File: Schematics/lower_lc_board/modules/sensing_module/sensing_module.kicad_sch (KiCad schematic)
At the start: 21 parts, among them J4 HALL-1, J5 HALL-2, Q3 2N7002, U11 SI2301CDS-T1-GE3, U9 ADC_ADS131M04IPWR

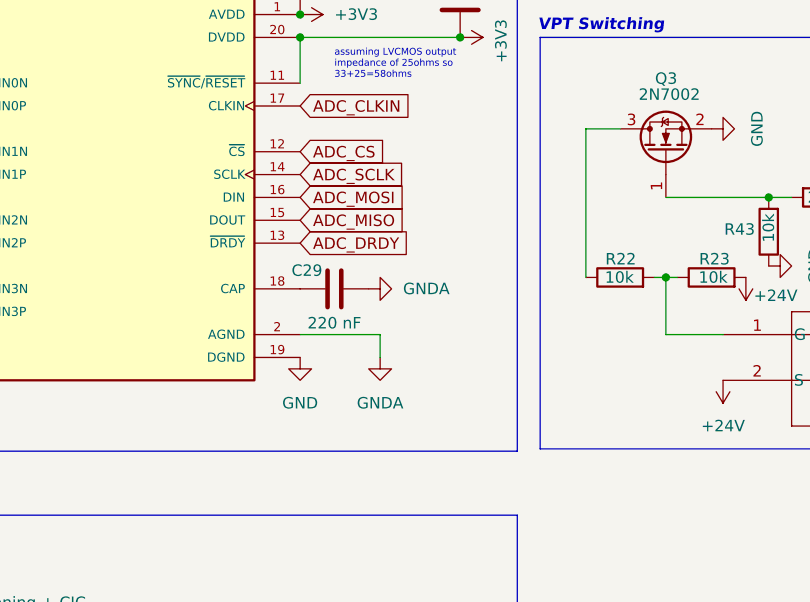
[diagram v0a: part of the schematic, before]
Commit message: routing work
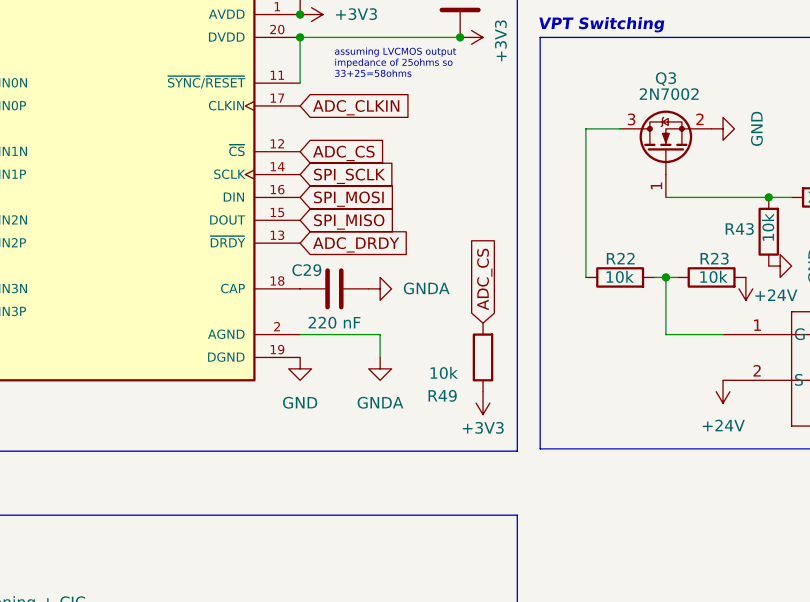
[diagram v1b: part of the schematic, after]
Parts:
- added R49: 10k, Resistor_SMD:R_0402_1005Metric, symbol Device:R
- C23, C33: JLCPCB (none) -> C49678
- J4, J5: footprint B04B_PASK_JST:CONN_B04B-PASK_JST -> S04B_PASK_2-P:CONN4_S04B-PASK_JST
- R22, R23: JLCPCB (none) -> C25744
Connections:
- net +3V3: now also R49.1
- net ADC_CS: now also R49.2
- net ADC_MISO renamed SPI_MISO
- net ADC_MOSI renamed SPI_MOSI
- net ADC_SCLK renamed SPI_SCLK
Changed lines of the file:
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@@
 		)
 	)
-	(global_label "ADC_DRDY"
+	(global_label "SPI_MISO"
 		(shape input)
-		(at 182.88 69.85 0)
+		(at 182.88 67.31 0)
 		(fields_autoplaced yes)
 		(effects
@@
 		)
 		(property "Intersheetrefs" "${INTERSHEET_REFS}"
-			(at 195.36 69.85 0)
+			(at 194.5133 67.31 0)
 			(effects
 				(font
@@
 		)
 	)
-	(global_label "HALL_SCL"
+	(global_label "ADC_DRDY"
 		(shape input)
-		(at 91.44 139.7 180)
+		(at 182.88 69.85 0)
 		(fields_autoplaced yes)
 		(effects
@@
 				(size 1.27 1.27)
 			)
-			(justify right)
+			(justify left)
 		)
 		(property "Intersheetrefs" "${INTERSHEET_REFS}"
-			(at 79.5043 139.7 0)
+			(at 195.36 69.85 0)
 			(effects
 				(font
 					(size 1.27 1.27)
 				)
-				(justify right)
+				(justify left)
 				(hide yes)
 			)
 		)
 	)
-	(global_label "ADC_CS"
+	(global_label "HALL_SCL"
 		(shape input)
-		(at 182.88 59.69 0)
+		(at 91.44 139.7 180)
 		(fields_autoplaced yes)
 		(effects
@@
 				(size 1.27 1.27)
 			)
-			(justify left)
+			(justify right)
 		)
 		(property "Intersheetrefs" "${INTERSHEET_REFS}"
-			(at 192.9409 59.69 0)
+			(at 79.5043 139.7 0)
 			(effects
 				(font
 					(size 1.27 1.27)
 				)
-				(justify left)
+				(justify right)
 				(hide yes)
 			)
 		)
 	)
-	(global_label "ADC_SCLK"
+	(global_label "ADC_CS"
 		(shape input)
-		(at 182.88 62.23 0)
+		(at 182.88 59.69 0)
 		(fields_autoplaced yes)
 		(effects
@@
 		)
 		(property "Intersheetrefs" "${INTERSHEET_REFS}"
-			(at 195.239 62.23 0)
+			(at 192.9409 59.69 0)
 			(effects
 				(font
@@
 		)
 	)
-	(global_label "ADC_MOSI"
+	(global_label "ADC_CLKIN"
 		(shape input)
-		(at 182.88 64.77 0)
+		(at 182.88 54.61 0)
 		(fields_autoplaced yes)
 		(effects
@@
 		)
 		(property "Intersheetrefs" "${INTERSHEET_REFS}"
-			(at 195.0576 64.77 0)
+			(at 195.9648 54.61 0)
 			(effects
 				(font
@@
 		)
 	)
-	(global_label "ADC_CLKIN"
+	(global_label "ADC_CS"
 		(shape input)
-		(at 182.88 54.61 0)
+		(at 203.2 78.74 90)
 		(fields_autoplaced yes)
 		(effects
@@
 		)
 		(property "Intersheetrefs" "${INTERSHEET_REFS}"
-			(at 195.9648 54.61 0)
+			(at 203.2 68.6791 90)
 			(effects
 				(font
@@
 		)
 	)
-	(global_label "ADC_MISO"
+	(global_label "SPI_SCLK"
 		(shape input)
-		(at 182.88 67.31 0)
+		(at 182.88 62.23 0)
 		(fields_autoplaced yes)
 		(effects
@@
 		)
 		(property "Intersheetrefs" "${INTERSHEET_REFS}"
-			(at 195.0576 67.31 0)
+			(at 194.6947 62.23 0)
 			(effects
 				(font
@@
 		)
 	)
+	(global_label "SPI_MOSI"
+		(shape input)
+		(at 182.88 64.77 0)
+		(fields_autoplaced yes)
+		(effects
+			(font
+				(size 1.27 1.27)
+			)
+			(justify left)
+		)
+		(property "Intersheetrefs" "${INTERSHEET_REFS}"
+			(at 194.5133 64.77 0)
+			(effects
+				(font
+					(size 1.27 1.27)
+				)
+				(justify left)
+				(hide yes)
+			)
+		)
+	)
 	(symbol
 		(lib_id "Device:C")
@@
 			)
 		)
+		(property "JLCPCB" "C25744"
+			(at 228.6 73.66 0)
+			(effects
+				(font
+					(size 1.27 1.27)
+				)
+				(hide yes)
+			)
+		)
 		(pin "1"
 		)
@@
 			)
 		)
+		(property "JLCPCB" "C49678"
+			(at 45.72 170.18 0)
+			(effects
+				(font
+					(size 1.27 1.27)
+				)
+				(hide yes)
+			)
+		)
 		(pin "2"
 		)
@@
 			)
 		)
-		(property "Footprint" "B04B_PASK_JST:CONN_B04B-PASK_JST"
+		(property "Footprint" "S04B_PASK_2-P:CONN4_S04B-PASK_JST"
 			(at 49.53 154.94 0)
 			(effects
@@
 			)
 		)
+		(property "JLCPCB" "C49678"
+			(at 45.72 130.81 0)
+			(effects
+				(font
+					(size 1.27 1.27)
+				)
+				(hide yes)
+			)
+		)
 		(pin "2"
 		)
@@
 	)
 	(symbol
+		(lib_id "power:+3V3")
+		(at 203.2 86.36 180)
+		(unit 1)
+		(exclude_from_sim no)
+		(in_bom yes)
+		(on_board yes)
+		(dnp no)
+		(property "Reference" "#PWR0132"
+			(at 203.2 82.55 0)
+			(effects
+				(font
+					(size 1.27 1.27)
+				)
+				(hide yes)
+			)
+		)
+		(property "Value" "+3V3"
+			(at 203.2 90.424 0)
+			(effects
+				(font
+					(size 1.27 1.27)
+				)
+			)
+		)
+		(property "Footprint" ""
+			(at 203.2 86.36 0)
+			(effects
+				(font
+					(size 1.27 1.27)
+				)
+				(hide yes)
+			)
+		)
+		(property "Datasheet" ""
+			(at 203.2 86.36 0)
+			(effects
+				(font
+					(size 1.27 1.27)
+				)
+				(hide yes)
+			)
+		)
+		(property "Description" "Power symbol creates a global label with name \"+3V3\""
+			(at 203.2 86.36 0)
+			(effects
+				(font
+					(size 1.27 1.27)
+				)
+				(hide yes)
+			)
+		)
+		(pin "1"
+		)
+		(instances
+			(project "lower_lc_board"
+				(path "/d63798c4-e363-437e-9012-e4aff32e6642/c6419db7-28a9-4bfa-8244-fc88166c795c"
+					(reference "#PWR0132")
+					(unit 1)
+				)
+			)
+		)
+	)
+	(symbol
 		(lib_id "Device:C")
 		(at 186.69 74.93 90)
@@
 			)
 		)
-		(property "Footprint" "B04B_PASK_JST:CONN_B04B-PASK_JST"
+		(property "Footprint" "S04B_PASK_2-P:CONN4_S04B-PASK_JST"
 			(at 49.53 115.57 0)
 			(effects
@@
 	(symbol
 		(lib_id "Device:R")
+		(at 203.2 82.55 180)
+		(unit 1)
+		(exclude_from_sim no)
+		(in_bom yes)
+		(on_board yes)
+		(dnp no)
+		(property "Reference" "R49"
+			(at 200.406 86.868 0)
+			(effects
+				(font
+					(size 1.27 1.27)
+				)
+				(justify left)
+			)
+		)
+		(property "Value" "10k"
+			(at 200.406 84.328 0)
+			(effects
+				(font
+					(size 1.27 1.27)
+				)
+				(justify left)
+			)
+		)
+		(property "Footprint" "Resistor_SMD:R_0402_1005Metric"
+			(at 204.978 82.55 90)
+			(effects
+				(font
+					(size 1.27 1.27)
+				)
+				(hide yes)
+			)
+		)
+		(property "Datasheet" "~"
+			(at 203.2 82.55 0)
+			(effects
+				(font
+					(size 1.27 1.27)
+				)
+				(hide yes)
+			)
+		)
+		(property "Description" "Resistor"
+			(at 203.2 82.55 0)
+			(effects
+				(font
+					(size 1.27 1.27)
+				)
+				(hide yes)
+			)
+		)
+		(property "JLCPCB" "C25744"
+			(at 203.2 82.55 0)
+			(effects
+				(font
+					(size 1.27 1.27)
+				)
+				(hide yes)
+			)
+		)
+		(pin "1"
+		)
+		(pin "2"
+		)
+		(instances
+			(project "lower_lc_board"
+				(path "/d63798c4-e363-437e-9012-e4aff32e6642/c6419db7-28a9-4bfa-8244-fc88166c795c"
+					(reference "R49")
+					(unit 1)
+				)
+			)
+		)
+	)
+	(symbol
+		(lib_id "Device:R")
 		(at 234.95 68.58 180)
 		(unit 1)
@@
 			(at 218.44 73.66 0)
 			(effects
+				(font
+					(size 1.27 1.27)
+				)
+				(hide yes)
+			)
+		)
+		(property "JLCPCB" "C25744"
+			(at 218.44 73.66 0)
+			(effects

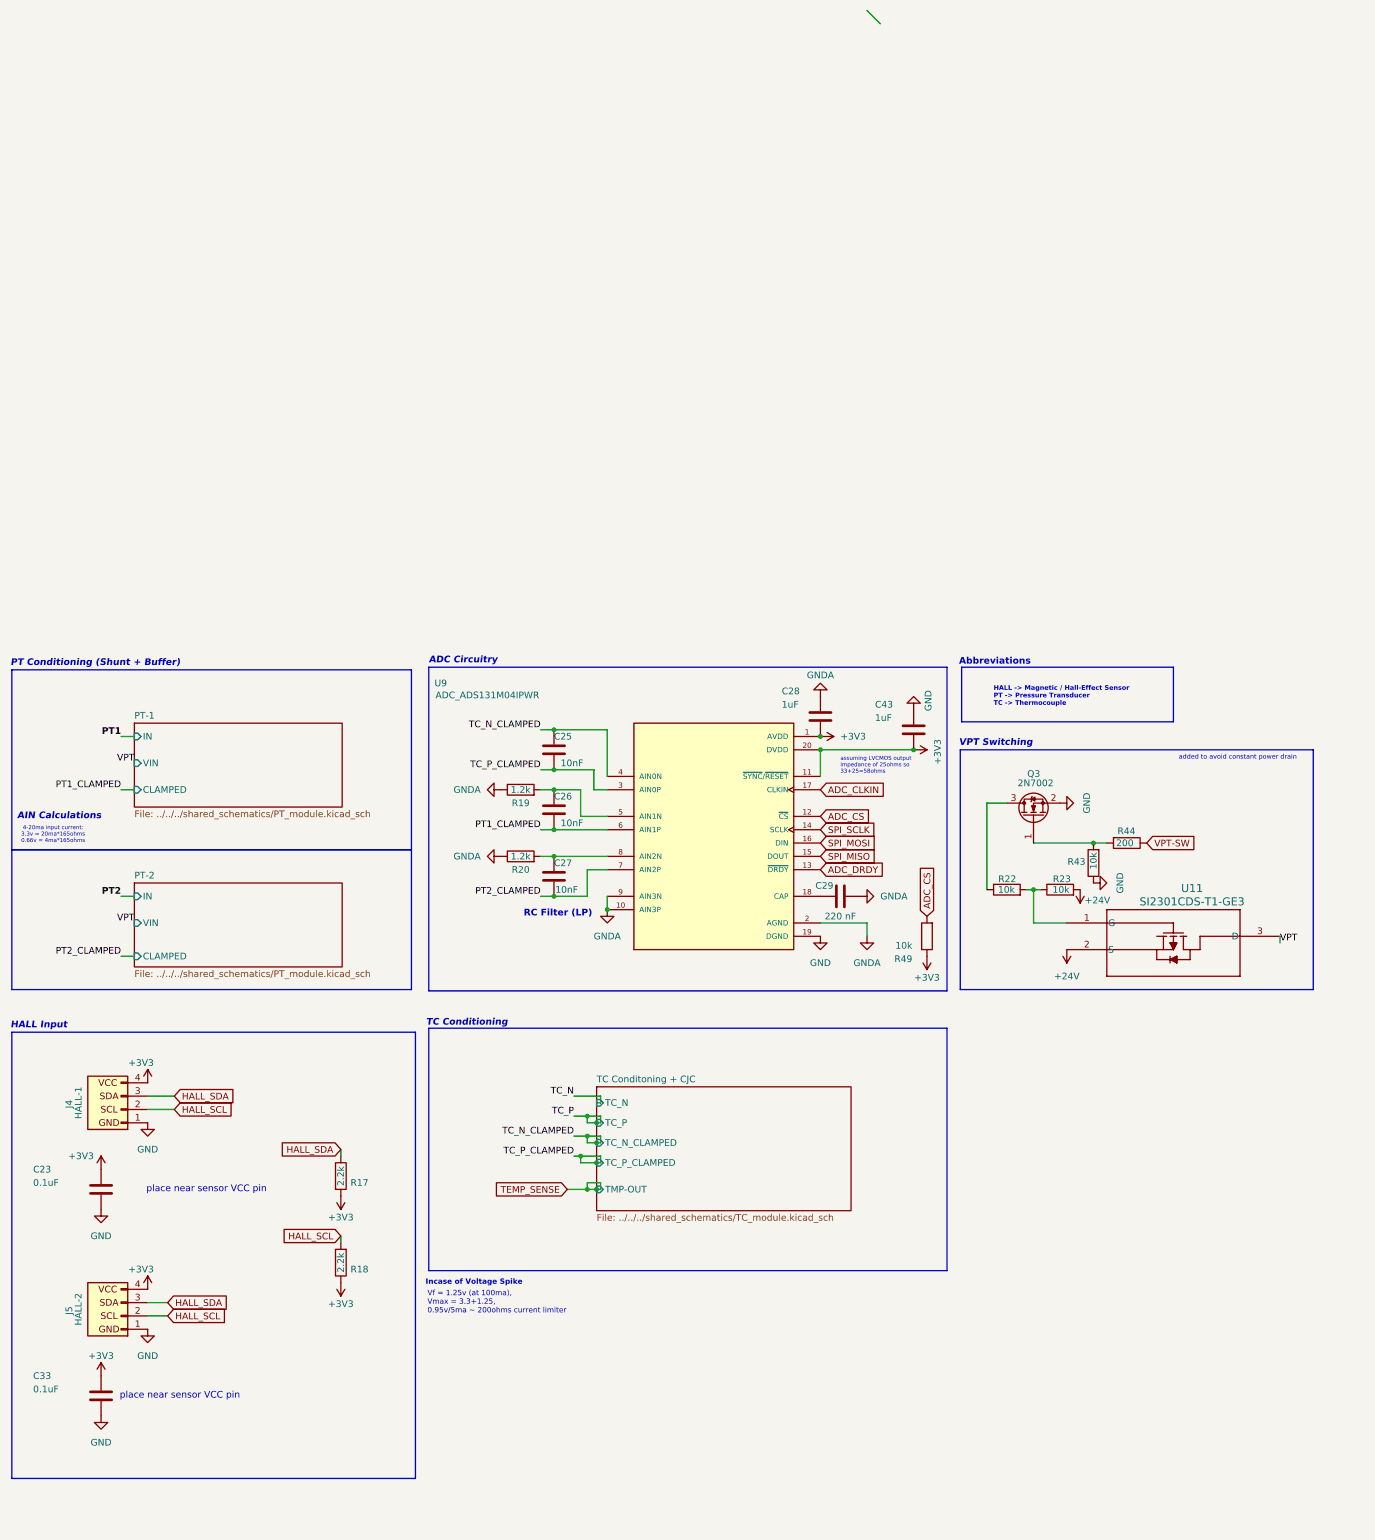
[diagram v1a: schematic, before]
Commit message: routing work
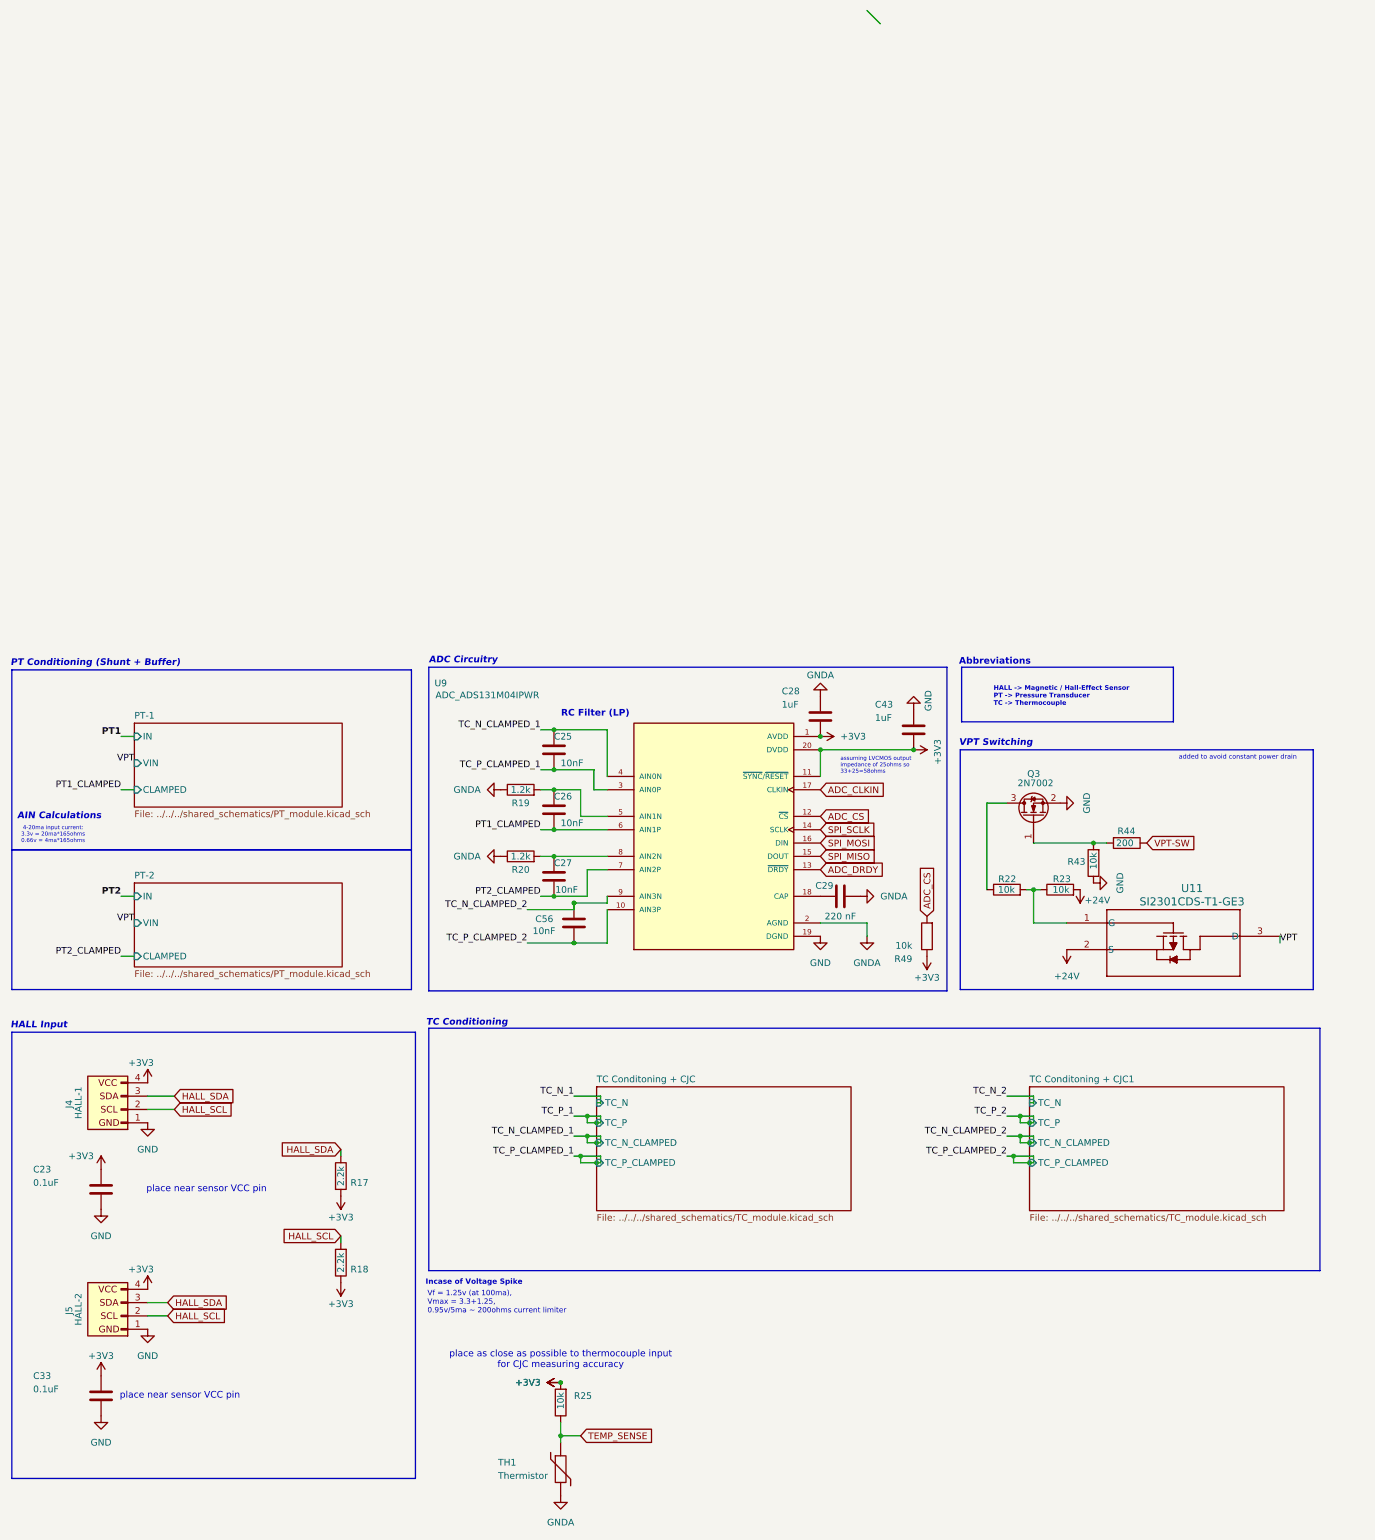
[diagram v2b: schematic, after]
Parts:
- added C56: 10nF, Capacitor_SMD:C_0603_1608Metric, symbol Device:C
- added R25: 10k, Resistor_SMD:R_0603_1608Metric, symbol Device:R
- added TH1: Thermistor, Resistor_SMD:R_0402_1005Metric, symbol Device:Thermistor
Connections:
- net +3V3: now also R25.2
- net GNDA: now also TH1.2; no longer U9.10 (AIN3P), U9.9 (AIN3N)
- net TEMP_SENSE: now also R25.1, TH1.1
- net TC_N_CLAMPED renamed TC_N_CLAMPED_1
- net TC_P_CLAMPED renamed TC_P_CLAMPED_1
- new net TC_N_CLAMPED_2: C56.1, U9.9 (AIN3N)
- new net TC_P_CLAMPED_2: C56.2, U9.10 (AIN3P)
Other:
- added sheet TC Conditoning + CJC1 (../../../shared_schematics/TC_module.kicad_sch)
- sheet TC Conditoning + CJC ports: added none; removed TMP-OUT
- note added: "place as close as possible to thermocouple input for CJC measuring accuracy"
